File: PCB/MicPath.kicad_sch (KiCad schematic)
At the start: 77 parts, among them J301 NC3FAH2, J302 Conn_01x02, J303 Conn_01x02, J304 Conn_01x02, J305 Conn_01x02, J306 NC3MAH, J307 NC3MAH, SW301 SW_SPST, SW302 SW_SPST, U301 TMUX6236, U302 OPA1678, U303 THAT1512, U304 THAT1646, U305 OPA202

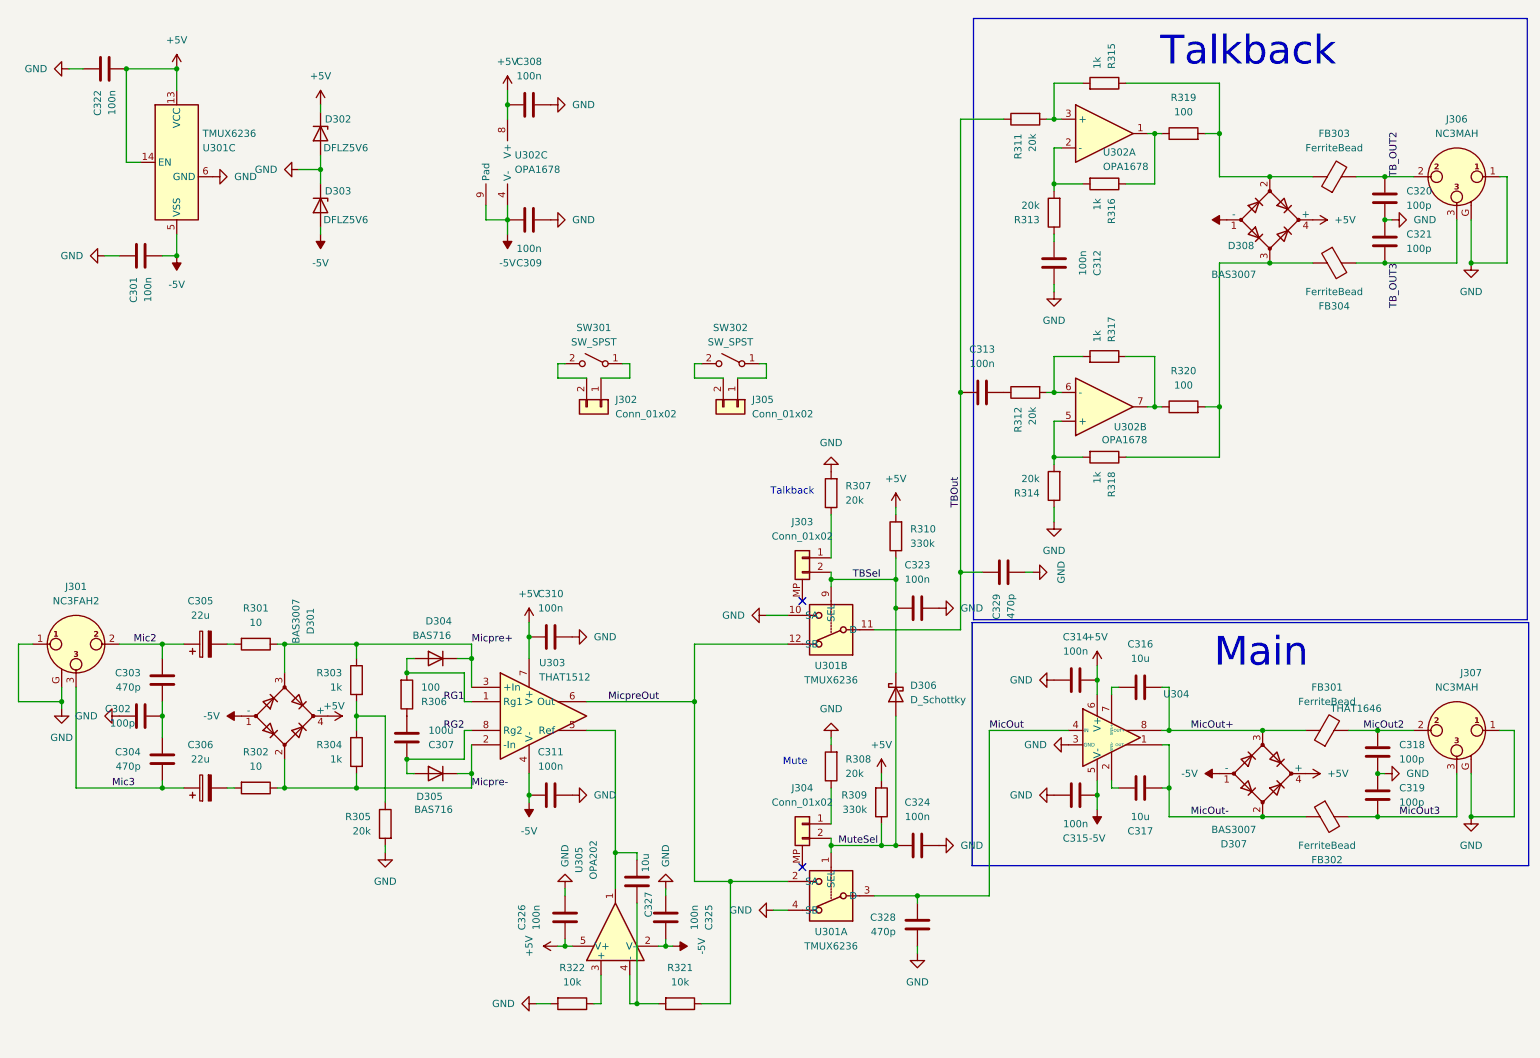
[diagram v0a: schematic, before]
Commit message: Tidying up
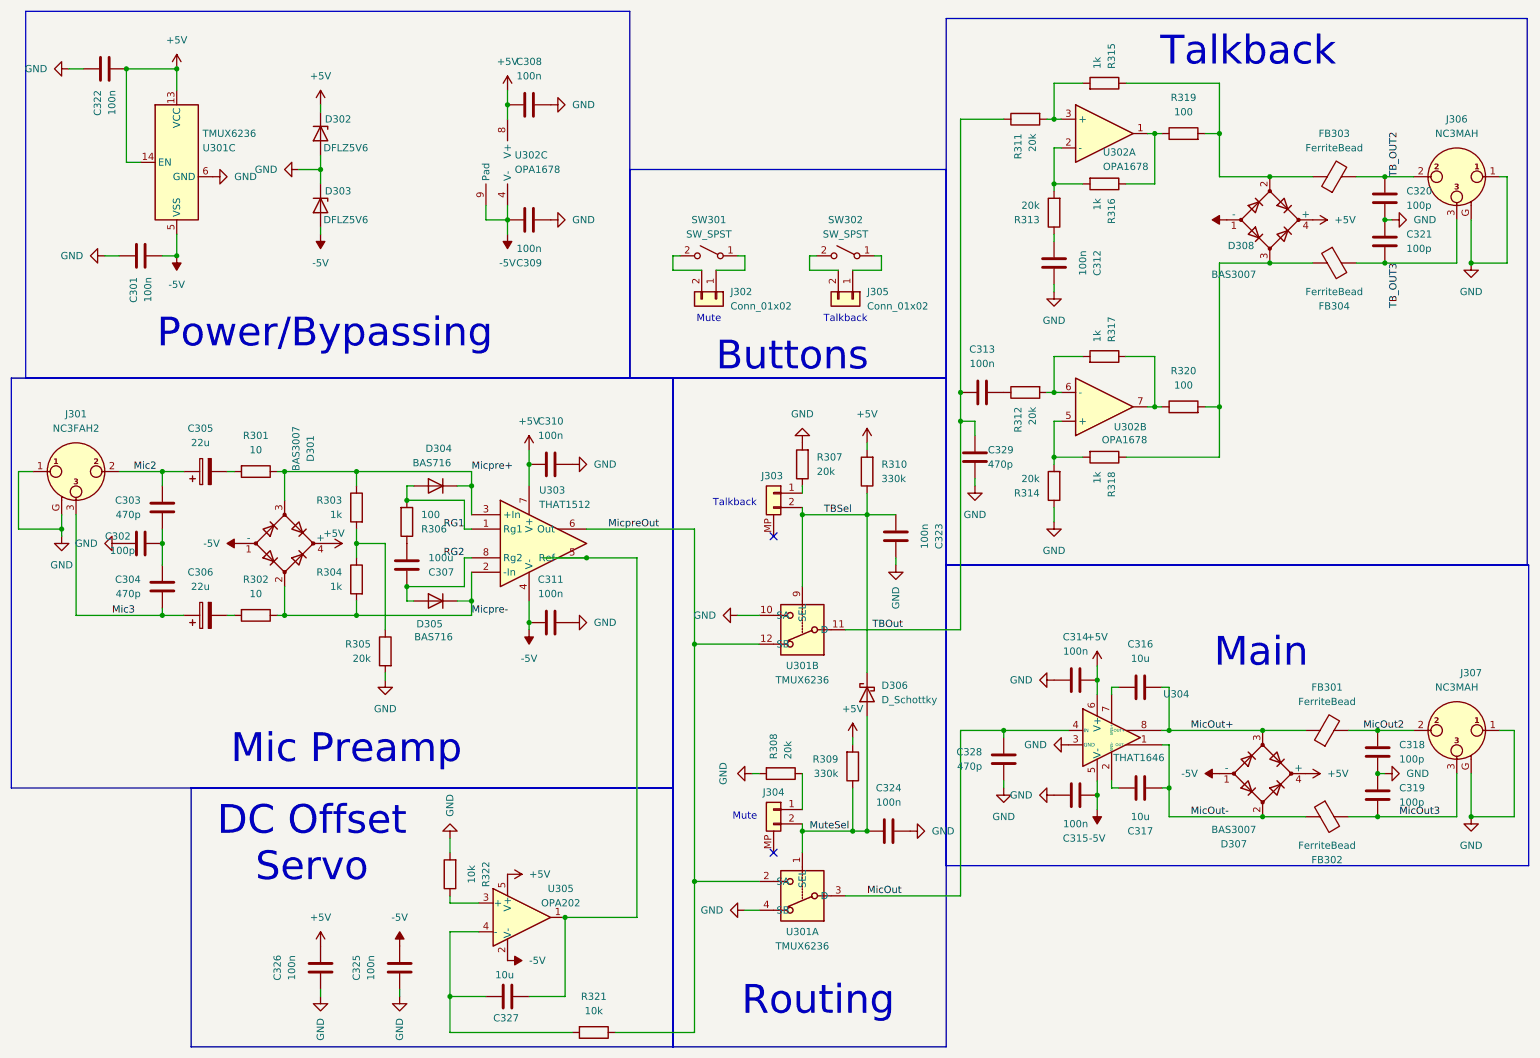
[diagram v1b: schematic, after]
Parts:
- U302: footprint STEVEannouncer:WSON-8-1EP_3x3mm_P0.5mm_EP1.2x2mm_ThermalVias -> Package_SON:WSON-8-1EP_3x3mm_P0.5mm_EP1.2x2mm_ThermalVias; Gearlabs Part Number (none) -> EXT-OPA1678
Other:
- note added: "Buttons"
- note added: "DC Offset Servo"
- note added: "Mic Preamp"
- note added: "Power/Bypassing"
- note added: "Routing"
- moved on the sheet: C302, C303, C304, C305, C306, C307, C310, C311, C323, C324, C325, C326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
